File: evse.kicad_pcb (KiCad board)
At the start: 2 copper layers, 100 x 100 mm, 119 parts, among them IC1 LF353, IC3 LM358, IC8 HCPL-2731S, J1 ISP, J4 T44009, J5 T44009, J6 T44009, J7 T44009, J8 T44009, J9 T44009, K1 HF186F/12-HCTF, K2 HF186F/12-HCTF, M1 MOV, M2 MOV, M3 MOV, Q2 MMBT2222A, Q3 MMBT2222A, U1 AP63205WU, U2 TC1044S, U3 MCP9808, U4 ATmega328P-AU, Y1 16MHz

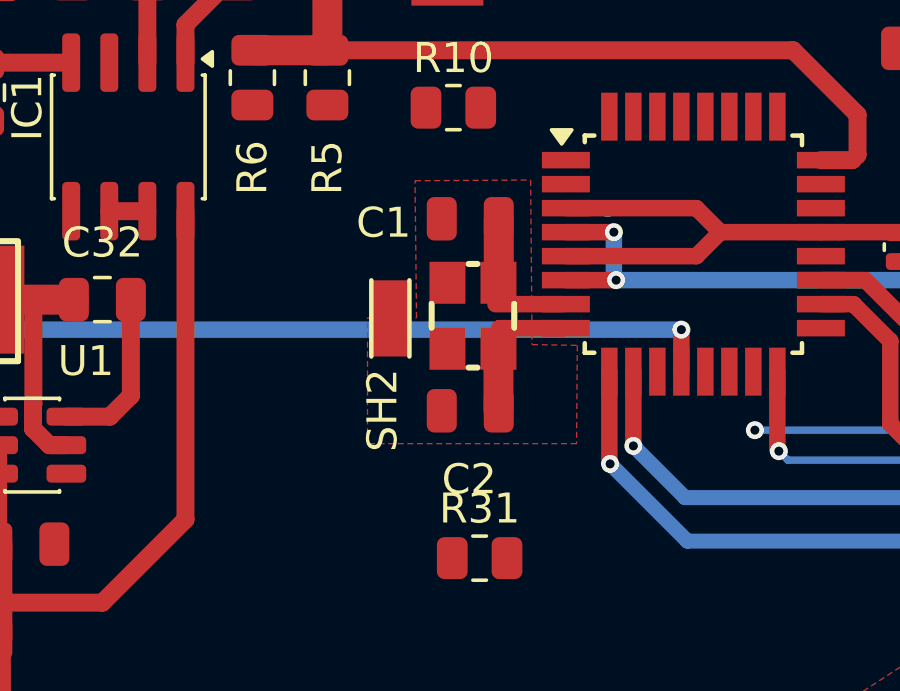
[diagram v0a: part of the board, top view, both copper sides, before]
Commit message: fix Y1
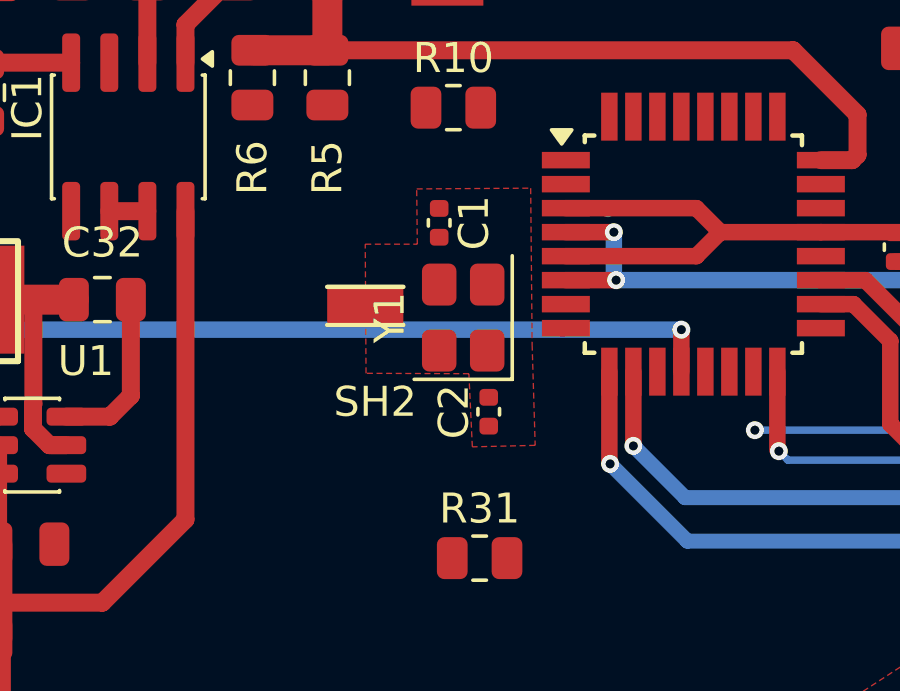
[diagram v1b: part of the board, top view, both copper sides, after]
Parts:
- C1, C2: value 22pF -> 12pF; footprint PCM_JLCPCB:C_0805 -> Capacitor_SMD:C_0402_1005Metric
- Y1: value 16MHz -> FA-238A 16MHz CL=8pF; footprint PCM_SparkFun-Clock:Crystal_SMD_3.2x2.5mm -> Crystal:Crystal_SMD_SeikoEpson_TSX3225-4Pin_3.2x2.5mm
- moved C1 1.04 mm to (69.6, 38.8), turned to -90 degrees
- moved SH2 0.93 mm to (67.1, 41.6), turned to 180 degrees
- moved C2 0.62 mm to (71.2, 45.1), turned to 90 degrees
- moved Y1 0.33 mm to (70.4, 41.9)
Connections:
- Y1 pad 2: Net-(U4-XTAL1/PB6) -> XGND
- Y1 pad 3: unconnected-(Y1-NC1-Pad3) -> Net-(U4-XTAL1/PB6)
- Y1 pad 4: unconnected-(Y1-NC2-Pad4) -> XGND
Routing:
- net Net-(U4-XTAL1/PB6): track 4.93 -> 0.00 mm
- net Net-(U4-XTAL2/PB7): track 4.85 -> 0.03 mm
